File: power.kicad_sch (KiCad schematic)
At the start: 27 parts, among them J201 Barrel_Jack_MountingPin, J204 Conn_01x04_f, Q201 AO4407C, U201 TPS54302, U202 AMS1117-3.3

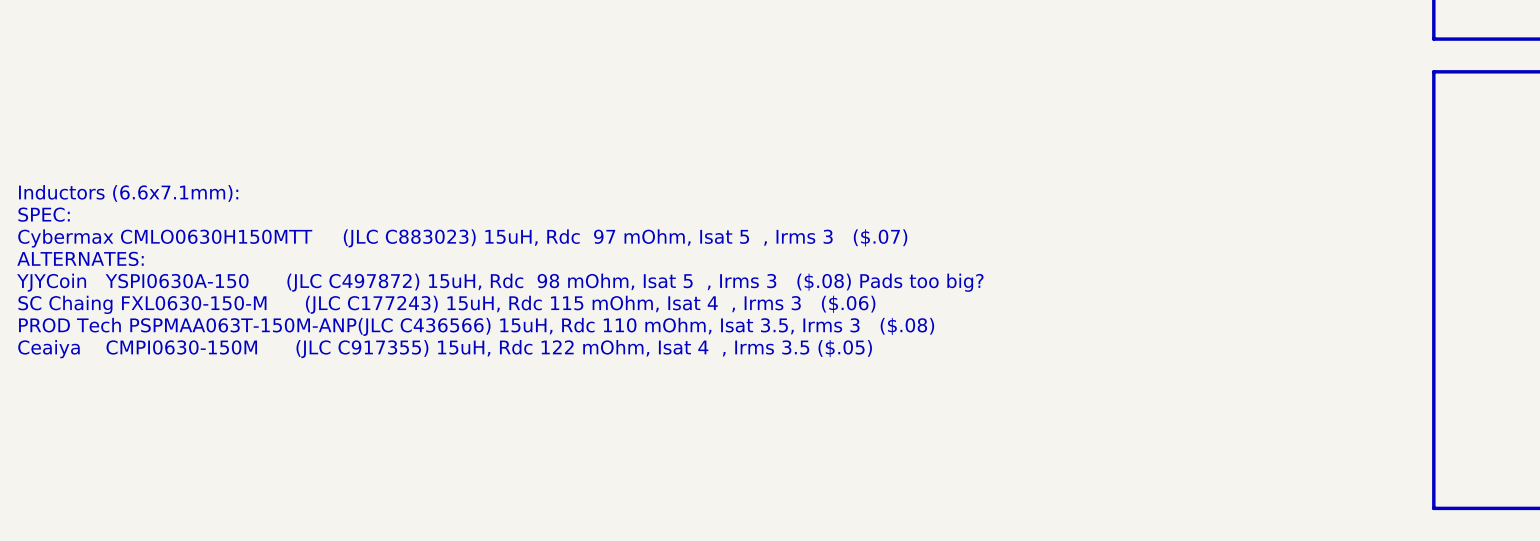
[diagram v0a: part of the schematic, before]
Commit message: Add files via upload
Update new inductor alternate
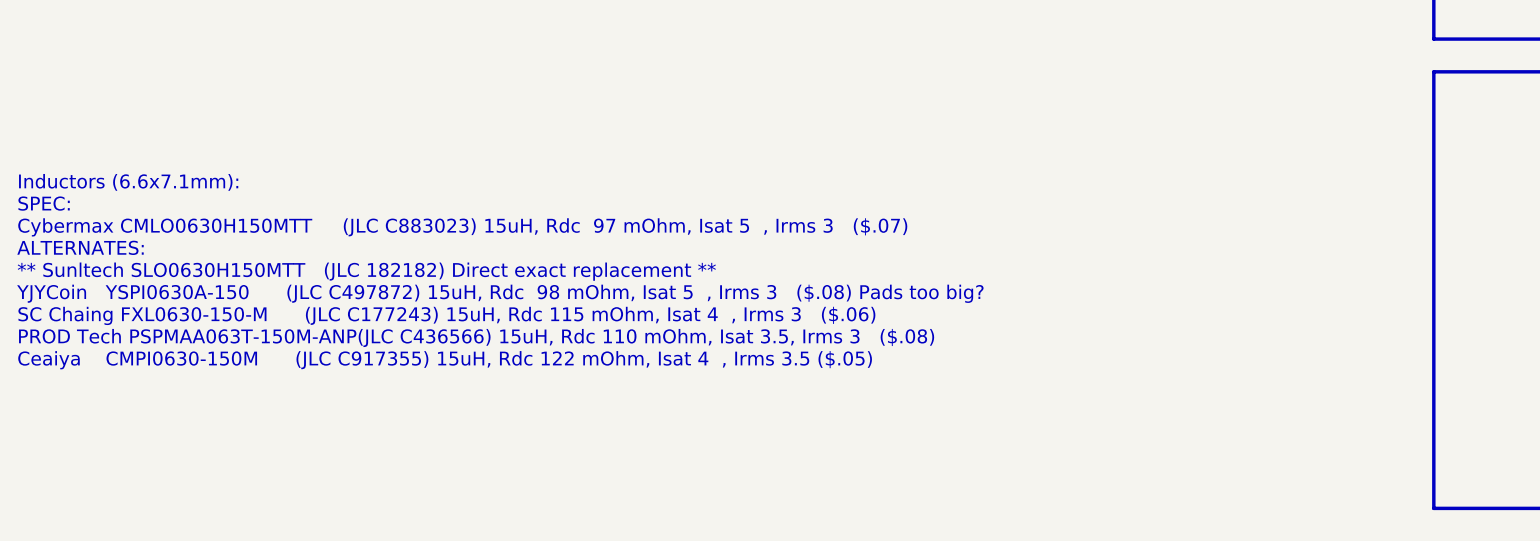
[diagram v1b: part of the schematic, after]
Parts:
- L201: Alternate C497872, C177243 -> C182182, C497872, C177243
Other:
- note added: "Inductors (6.6x7.1mm): SPEC: Cybermax CMLO0630H150MTT (JLC C883023) 15uH, Rdc 97 mOhm, Isat 5 , Irms 3 ($.07) ALTERNATES: ** Sunltech SLO0630H150MTT (JLC 182182) Direct exact replacement ** YJYCoin YSPI0630A-150 (JLC C497872) 15uH, Rdc 98 mOhm, Isat 5 , Irms 3 ($.08) Pads too big? SC Chaing FXL0630-150-M (JLC C177243) 15uH, Rdc 115 mOhm, Isat 4 , Irms 3 ($.06) PROD Tech PSPMAA063T-150M-ANP(JLC C4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"
- note removed: "Inductors (6.6x7.1mm): SPEC: Cybermax CMLO0630H150MTT (JLC C883023) 15uH, Rdc 97 mOhm, Isat 5 , Irms 3 ($.07) ALTERNATES: YJYCoin YSPI0630A-150 (JLC C497872) 15uH, Rdc 98 mOhm, Isat 5 , Irms 3 ($.08) Pads too big? SC Chaing FXL0630-150-M (JLC C177243) 15uH, Rdc 115 mOhm, Isat 4 , Irms 3 ($.06) PROD Tech PSPMAA063T-150M-ANP(JLC C436566) 15uH, Rdc 110 mOhm, Isat 3.5, Irms 3 ($.08) Ceaiya CMPI0630-1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"
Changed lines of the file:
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@@
 		)
 	)
-	(text "Inductors (6.6x7.1mm):\nSPEC: \nCybermax CMLO0630H150MTT     (JLC C883023) 15uH, Rdc  97 mOhm, Isat 5  , Irms 3   ($.07)\nALTERNATES:\nYJYCoin   YSPI0630A-150      (JLC C497872) 15uH, Rdc  98 mOhm, Isat 5  , Irms 3   ($.08) Pads too big?\nSC Chaing FXL0630-150-M      (JLC C177243) 15uH, Rdc 115 mOhm, Isat 4  , Irms 3   ($.06)\nPROD Tech PSPMAA063T-150M-ANP(JLC C436566) 15uH, Rdc 110 mOhm, Isat 3.5, Irms 3   ($.08)\nCeaiya    CMPI0630-150M      (JLC C917355) 15uH, Rdc 122 mOhm, Isat 4  , Irms 3.5 ($.05)"
+	(text "Inductors (6.6x7.1mm):\nSPEC: \nCybermax CMLO0630H150MTT     (JLC C883023) 15uH, Rdc  97 mOhm, Isat 5  , Irms 3   ($.07)\nALTERNATES:\n** Sunltech SLO0630H150MTT   (JLC 182182) Direct exact replacement **\nYJYCoin   YSPI0630A-150      (JLC C497872) 15uH, Rdc  98 mOhm, Isat 5  , Irms 3   ($.08) Pads too big?\nSC Chaing FXL0630-150-M      (JLC C177243) 15uH, Rdc 115 mOhm, Isat 4  , Irms 3   ($.06)\nPROD Tech PSPMAA063T-150M-ANP(JLC C436566) 15uH, Rdc 110 mOhm, Isat 3.5, Irms 3   ($.08)\nCeaiya    CMPI0630-150M      (JLC C917355) 15uH, Rdc 122 mOhm, Isat 4  , Irms 3.5 ($.05)"
 		(exclude_from_sim no)
 		(at -141.986 93.218 0)
@@
 			)
 		)
-		(property "Alternate" "C497872, C177243"
+		(property "Alternate" "C182182, C497872, C177243"
 			(at 170.18 86.36 90)
 			(effects

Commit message: Add reseller silkcreen files and add alternate parts numbers
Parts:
- C201, C202, C203: Alternate (none) -> C72478
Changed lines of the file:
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@@
+			)
+		)
+		(property "Alternate" "C72478"
+			(at 182.88 44.45 0)
+			(effects
+				(font
+					(size 1.27 1.27)
+				)
+				(hide yes)
 			)
 		)
@@
 			)
 		)
+		(property "Alternate" "C72478"
+			(at 196.85 44.45 0)
+			(effects
+				(font
+					(size 1.27 1.27)
+				)
+				(hide yes)
+			)
+		)
 		(pin "1"
 		)
@@
 			(at 210.82 44.45 0)
 			(effects
+				(font
+					(size 1.27 1.27)
+				)
+				(hide yes)
+			)
+		)
+		(property "Alternate" "C72478"
+			(at 210.82 44.45 0)
+			(effects
